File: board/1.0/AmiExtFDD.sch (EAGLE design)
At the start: 17 parts, among them J1 READY, J2 DISK CHANGE, J3 DSx Number, J4 DFx Number, J5 HD/DD, U1 74LS74, U2 74LS38

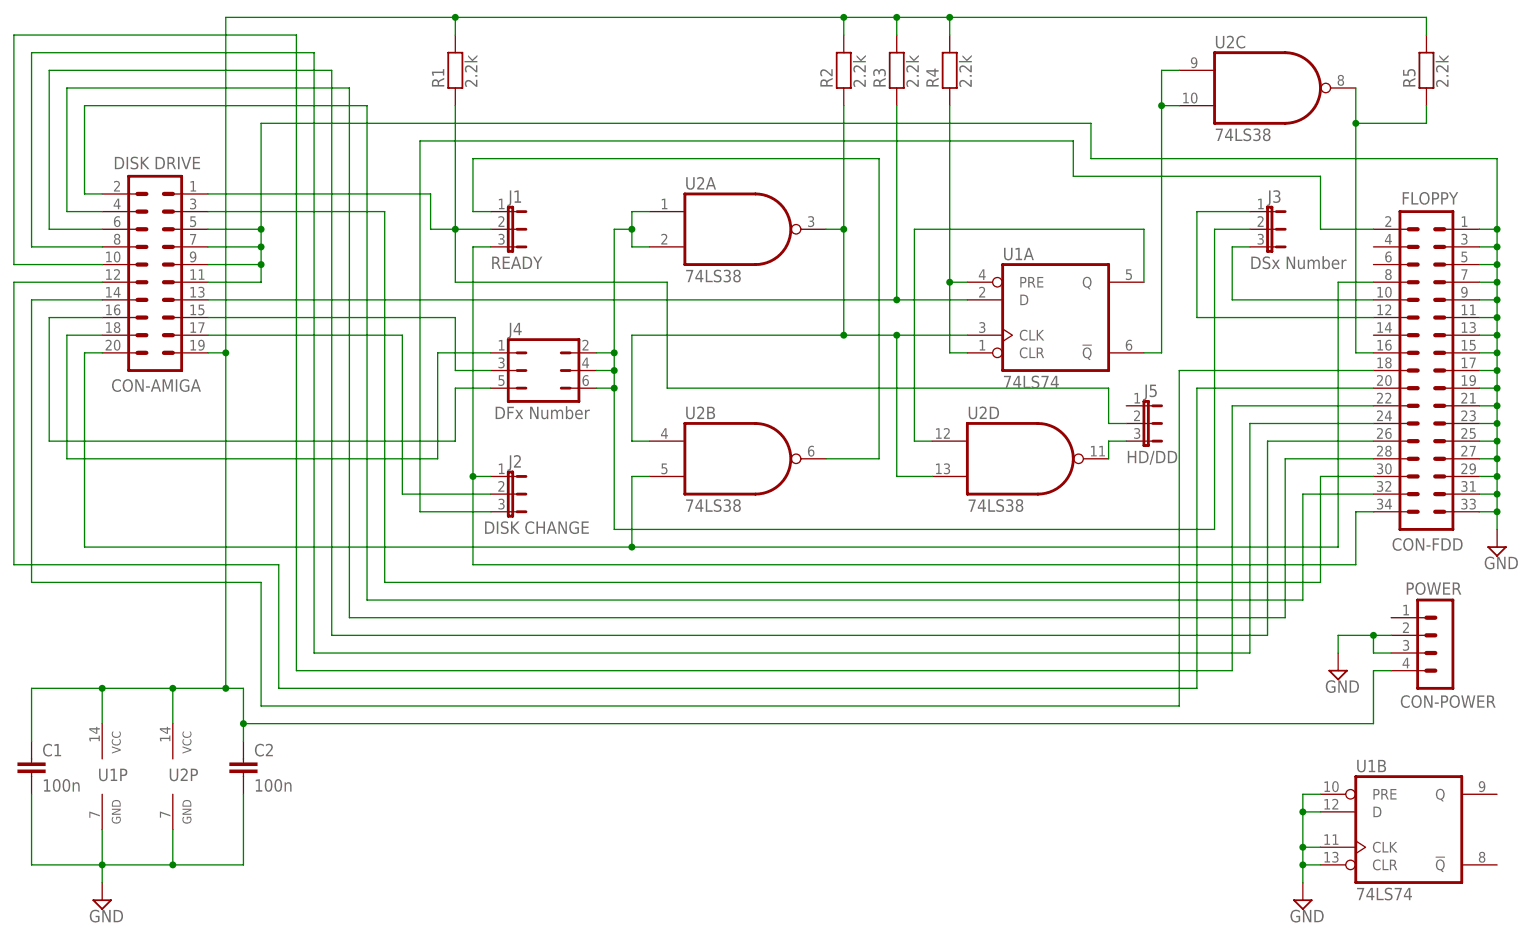
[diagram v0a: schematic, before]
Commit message: Little change on board and scheme
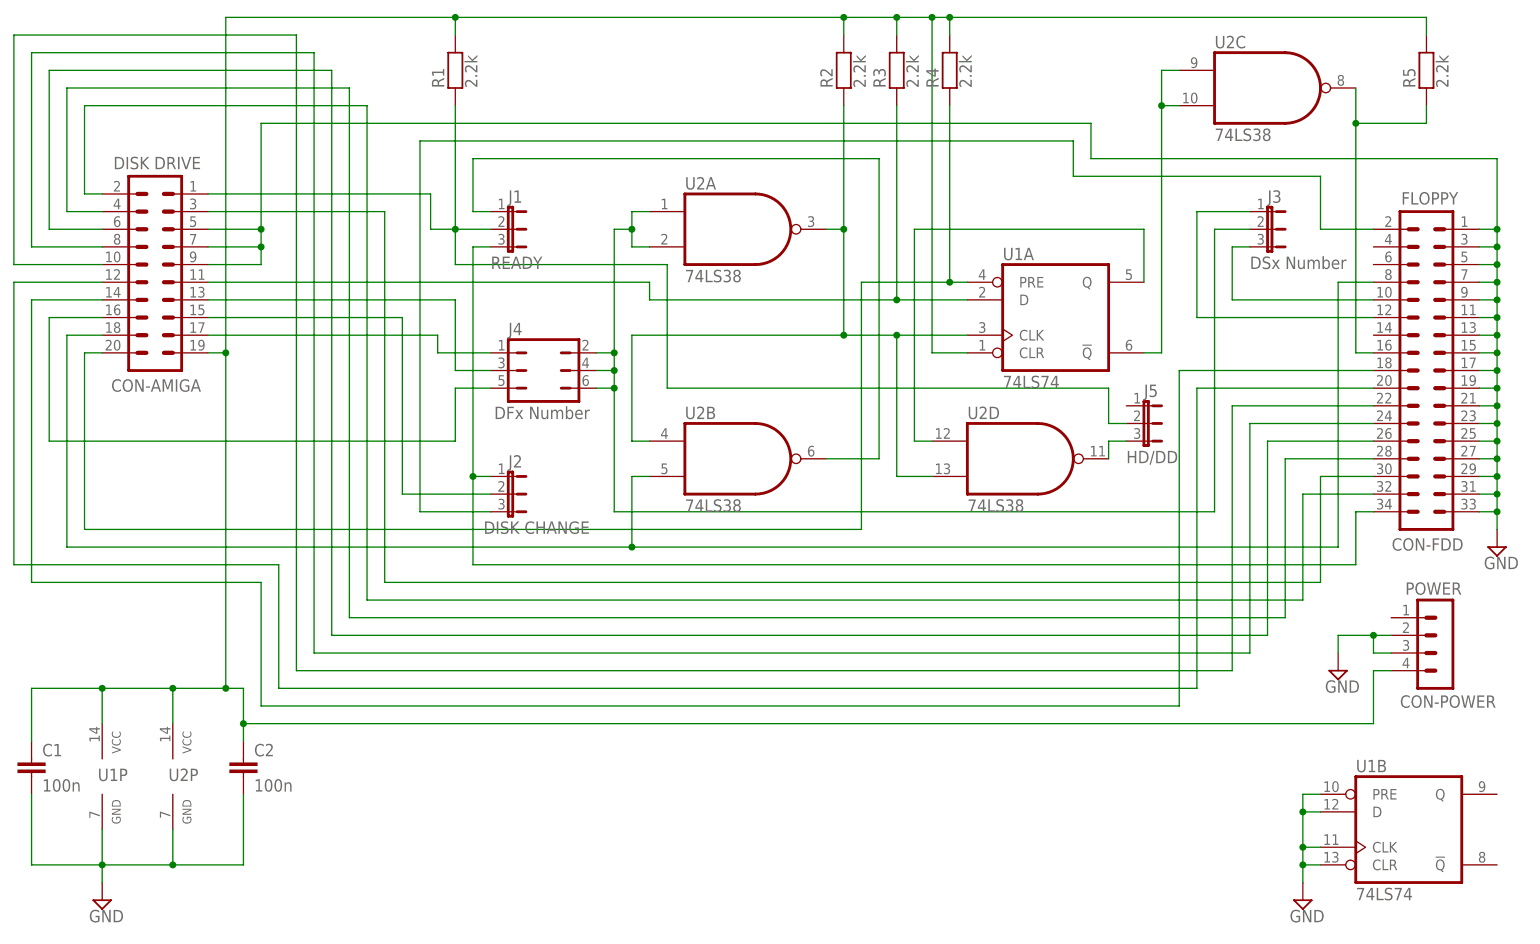
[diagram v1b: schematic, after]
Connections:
- removed net N$14: CON-AMIGA.18, J4.1
- new net N$7: CON-AMIGA.17, J4.1
- net GND: no longer CON-AMIGA.11
- net N$1: now also CON-AMIGA.15; no longer CON-AMIGA.17
- net N$15: now also CON-AMIGA.13; no longer CON-AMIGA.15
- net N$21: now also CON-AMIGA.18; no longer CON-AMIGA.20
- net N$24: now also CON-AMIGA.11; no longer CON-AMIGA.13
- net N$25: now also U1A.CLR
- net N$33: now also CON-AMIGA.20; no longer U1A.CLR
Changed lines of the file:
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@@
 <wire x1="-124.46" y1="43.18" x2="-124.46" y2="40.64" width="0.1524" layer="91"/>
 <wire x1="-124.46" y1="40.64" x2="-124.46" y2="38.1" width="0.1524" layer="91"/>
-<wire x1="-124.46" y1="38.1" x2="-124.46" y2="35.56" width="0.1524" layer="91"/>
-<wire x1="-132.08" y1="35.56" x2="-124.46" y2="35.56" width="0.1524" layer="91"/>
 <wire x1="-132.08" y1="38.1" x2="-124.46" y2="38.1" width="0.1524" layer="91"/>
 <wire x1="-132.08" y1="40.64" x2="-124.46" y2="40.64" width="0.1524" layer="91"/>
@@
 <junction x="53.34" y="5.08"/>
 <junction x="53.34" y="2.54"/>
-<junction x="-124.46" y="38.1"/>
 <junction x="-124.46" y="40.64"/>
 <junction x="-124.46" y="43.18"/>
@@
 <pinref part="CON-AMIGA" gate="G$1" pin="7"/>
 <pinref part="CON-AMIGA" gate="G$1" pin="9"/>
-<pinref part="CON-AMIGA" gate="G$1" pin="11"/>
 </segment>
 <segment>
@@
 <net name="N$1" class="0">
 <segment>
-<wire x1="-104.14" y1="27.94" x2="-104.14" y2="5.08" width="0.1524" layer="91"/>
+<wire x1="-104.14" y1="30.48" x2="-104.14" y2="5.08" width="0.1524" layer="91"/>
 <wire x1="-104.14" y1="5.08" x2="-91.44" y2="5.08" width="0.1524" layer="91"/>
-<wire x1="-132.08" y1="27.94" x2="-104.14" y2="27.94" width="0.1524" layer="91"/>
 <pinref part="J2" gate="G$1" pin="2"/>
-<pinref part="CON-AMIGA" gate="G$1" pin="17"/>
+<pinref part="CON-AMIGA" gate="G$1" pin="15"/>
+<wire x1="-132.08" y1="30.48" x2="-104.14" y2="30.48" width="0.1524" layer="91"/>
 </segment>
 </net>
@@
 </segment>
 </net>
-<net name="N$14" class="0">
-<segment>
-<wire x1="-99.06" y1="10.16" x2="-99.06" y2="25.4" width="0.1524" layer="91"/>
-<wire x1="-99.06" y1="25.4" x2="-91.44" y2="25.4" width="0.1524" layer="91"/>
-<wire x1="-152.4" y1="10.16" x2="-99.06" y2="10.16" width="0.1524" layer="91"/>
-<wire x1="-152.4" y1="10.16" x2="-152.4" y2="27.94" width="0.1524" layer="91"/>
-<wire x1="-152.4" y1="27.94" x2="-147.32" y2="27.94" width="0.1524" layer="91"/>
-<pinref part="J4" gate="G$1" pin="1"/>
-<pinref part="CON-AMIGA" gate="G$1" pin="18"/>
-</segment>
-</net>
 <net name="N$15" class="0">
 <segment>
-<wire x1="-96.52" y1="30.48" x2="-96.52" y2="22.86" width="0.1524" layer="91"/>
+<wire x1="-96.52" y1="33.02" x2="-96.52" y2="22.86" width="0.1524" layer="91"/>
 <wire x1="-96.52" y1="22.86" x2="-91.44" y2="22.86" width="0.1524" layer="91"/>
-<wire x1="-132.08" y1="30.48" x2="-96.52" y2="30.48" width="0.1524" layer="91"/>
 <pinref part="J4" gate="G$1" pin="3"/>
-<pinref part="CON-AMIGA" gate="G$1" pin="15"/>
+<pinref part="CON-AMIGA" gate="G$1" pin="13"/>
+<wire x1="-132.08" y1="33.02" x2="-96.52" y2="33.02" width="0.1524" layer="91"/>
 </segment>
 </net>
@@
 <wire x1="-76.2" y1="20.32" x2="-73.66" y2="20.32" width="0.1524" layer="91"/>
 <wire x1="-73.66" y1="20.32" x2="-73.66" y2="22.86" width="0.1524" layer="91"/>
-<wire x1="-73.66" y1="0" x2="-73.66" y2="20.32" width="0.1524" layer="91"/>
-<wire x1="12.7" y1="0" x2="-73.66" y2="0" width="0.1524" layer="91"/>
+<wire x1="-73.66" y1="2.54" x2="-73.66" y2="20.32" width="0.1524" layer="91"/>
+<wire x1="12.7" y1="2.54" x2="-73.66" y2="2.54" width="0.1524" layer="91"/>
 <wire x1="12.7" y1="43.18" x2="17.78" y2="43.18" width="0.1524" layer="91"/>
-<wire x1="12.7" y1="43.18" x2="12.7" y2="0" width="0.1524" layer="91"/>
+<wire x1="12.7" y1="43.18" x2="12.7" y2="2.54" width="0.1524" layer="91"/>
 <wire x1="-73.66" y1="25.4" x2="-73.66" y2="43.18" width="0.1524" layer="91"/>
 <wire x1="-68.58" y1="40.64" x2="-71.12" y2="40.64" width="0.1524" layer="91"/>
@@
 <wire x1="-71.12" y1="7.62" x2="-68.58" y2="7.62" width="0.1524" layer="91"/>
 <wire x1="-71.12" y1="7.62" x2="-71.12" y2="-2.54" width="0.1524" layer="91"/>
-<wire x1="-149.86" y1="-2.54" x2="-71.12" y2="-2.54" width="0.1524" layer="91"/>
+<wire x1="-152.4" y1="-2.54" x2="-71.12" y2="-2.54" width="0.1524" layer="91"/>
 <wire x1="-71.12" y1="-2.54" x2="30.48" y2="-2.54" width="0.1524" layer="91"/>
-<wire x1="-147.32" y1="25.4" x2="-149.86" y2="25.4" width="0.1524" layer="91"/>
-<wire x1="-149.86" y1="25.4" x2="-149.86" y2="-2.54" width="0.1524" layer="91"/>
 <junction x="-71.12" y="-2.54"/>
 <pinref part="U2" gate="B" pin="I1"/>
 <pinref part="CON-FDD" gate="G$1" pin="8"/>
-<pinref part="CON-AMIGA" gate="G$1" pin="20"/>
+<pinref part="CON-AMIGA" gate="G$1" pin="18"/>
+<wire x1="-147.32" y1="27.94" x2="-152.4" y2="27.94" width="0.1524" layer="91"/>
+<wire x1="-152.4" y1="27.94" x2="-152.4" y2="-2.54" width="0.1524" layer="91"/>
 </segment>
 </net>
@@
 <pinref part="J1" gate="G$1" pin="2"/>
 <pinref part="CON-AMIGA" gate="G$1" pin="1"/>
-<wire x1="-96.52" y1="43.18" x2="-96.52" y2="35.56" width="0.1524" layer="91"/>
-<wire x1="-96.52" y1="35.56" x2="-66.04" y2="35.56" width="0.1524" layer="91"/>
+<wire x1="-96.52" y1="43.18" x2="-96.52" y2="38.1" width="0.1524" layer="91"/>
+<wire x1="-96.52" y1="38.1" x2="-66.04" y2="38.1" width="0.1524" layer="91"/>
 <junction x="-96.52" y="43.18"/>
-<wire x1="-66.04" y1="35.56" x2="-66.04" y2="20.32" width="0.1524" layer="91"/>
+<wire x1="-66.04" y1="38.1" x2="-66.04" y2="20.32" width="0.1524" layer="91"/>
 <pinref part="R1" gate="G$1" pin="1"/>
 <wire x1="-96.52" y1="60.96" x2="-96.52" y2="43.18" width="0.1524" layer="91"/>
@@
 <wire x1="-33.02" y1="33.02" x2="-22.86" y2="33.02" width="0.1524" layer="91"/>
 <wire x1="-33.02" y1="33.02" x2="-33.02" y2="60.96" width="0.1524" layer="91"/>
-<wire x1="-132.08" y1="33.02" x2="-33.02" y2="33.02" width="0.1524" layer="91"/>
 <junction x="-33.02" y="33.02"/>
 <pinref part="R3" gate="G$1" pin="1"/>
 <pinref part="U1" gate="A" pin="D"/>
-<pinref part="CON-AMIGA" gate="G$1" pin="13"/>
+<pinref part="CON-AMIGA" gate="G$1" pin="11"/>
+<wire x1="-68.58" y1="33.02" x2="-33.02" y2="33.02" width="0.1524" layer="91"/>
+<wire x1="-132.08" y1="35.56" x2="-68.58" y2="35.56" width="0.1524" layer="91"/>
+<wire x1="-68.58" y1="35.56" x2="-68.58" y2="33.02" width="0.1524" layer="91"/>
 </segment>
 </net>
@@
 <wire x1="-96.52" y1="73.66" x2="-40.64" y2="73.66" width="0.1524" layer="91"/>
 <wire x1="-40.64" y1="73.66" x2="-33.02" y2="73.66" width="0.1524" layer="91"/>
-<wire x1="-33.02" y1="73.66" x2="-25.4" y2="73.66" width="0.1524" layer="91"/>
+<wire x1="-33.02" y1="73.66" x2="-27.94" y2="73.66" width="0.1524" layer="91"/>
+<wire x1="-27.94" y1="73.66" x2="-25.4" y2="73.66" width="0.1524" layer="91"/>
 <wire x1="-25.4" y1="73.66" x2="-25.4" y2="71.12" width="0.1524" layer="91"/>
 <wire x1="-33.02" y1="71.12" x2="-33.02" y2="73.66" width="0.1524" layer="91"/>
@@
 <wire x1="-96.52" y1="71.12" x2="-96.52" y2="73.66" width="0.1524" layer="91"/>
 <junction x="-96.52" y="73.66"/>
+<pinref part="U1" gate="A" pin="CLR"/>
+<wire x1="-22.86" y1="25.4" x2="-27.94" y2="25.4" width="0.1524" layer="91"/>
+<wire x1="-27.94" y1="25.4" x2="-27.94" y2="73.66" width="0.1524" layer="91"/>
+<junction x="-27.94" y="73.66"/>
 </segment>
 </net>
@@
 <net name="N$33" class="0">
 <segment>
-<wire x1="-22.86" y1="25.4" x2="-25.4" y2="25.4" width="0.1524" layer="91"/>
-<wire x1="-25.4" y1="25.4" x2="-25.4" y2="35.56" width="0.1524" layer="91"/>
 <wire x1="-25.4" y1="35.56" x2="-22.86" y2="35.56" width="0.1524" layer="91"/>
 <wire x1="-25.4" y1="35.56" x2="-25.4" y2="60.96" width="0.1524" layer="91"/>
+<pinref part="R4" gate="G$1" pin="1"/>
+<pinref part="U1" gate="A" pin="PRE"/>
+<wire x1="-25.4" y1="35.56" x2="-38.1" y2="35.56" width="0.1524" layer="91"/>
+<wire x1="-38.1" y1="35.56" x2="-38.1" y2="0" width="0.1524" layer="91"/>
 <junction x="-25.4" y="35.56"/>
-<pinref part="R4" gate="G$1" pin="1"/>
-<pinref part="U1" gate="A" pin="CLR"/>
-<pinref part="U1" gate="A" pin="PRE"/>
+<wire x1="-38.1" y1="0" x2="-149.86" y2="0" width="0.1524" layer="91"/>
+<wire x1="-149.86" y1="0" x2="-149.86" y2="25.4" width="0.1524" layer="91"/>
+<pinref part="CON-AMIGA" gate="G$1" pin="20"/>
+<wire x1="-149.86" y1="25.4" x2="-147.32" y2="25.4" width="0.1524" layer="91"/>
 </segment>
 </net>
@@
 </segment>
 </net>
+<net name="N$7" class="0">
+<segment>
+<pinref part="CON-AMIGA" gate="G$1" pin="17"/>
+<wire x1="-132.08" y1="27.94" x2="-99.06" y2="27.94" width="0.1524" layer="91"/>
+<wire x1="-99.06" y1="27.94" x2="-99.06" y2="25.4" width="0.1524" layer="91"/>
+<wire x1="-99.06" y1="25.4" x2="-91.44" y2="25.4" width="0.1524" layer="91"/>
+<pinref part="J4" gate="G$1" pin="1"/>
+</segment>
+</net>
